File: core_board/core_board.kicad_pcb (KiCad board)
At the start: 2 copper layers, 101.6 x 113.2 mm, 111 parts, among them J1 Molex_Megafit_02, J10 Conn_01x04_Pin, J11 Conn_01x02_Pin, J12 Conn_01x02_Pin, J13 Conn_01x03_Pin, J14 Conn_01x02_Pin, J15 Conn_01x02_Pin, J16 Conn_01x03_Pin, J2 RJ45_LED_Shielded, J3 Conn_01x02_Pin, J4Serv1 Conn_01x04_Pin, J5 Conn_01x04_Pin, J6 Conn_01x02_Pin, J8 Conn_01x04_Pin, J9 Conn_01x02_Pin, Q1 TPC8132_LQS, Q18 BSS138, Q19 BSS138, Q2 BSS138, Q20 BSS138, Q21 BSS138, Q3 BSS138, Q4 BSS138, Q5 BSS138, Q6 BSS138, Q7 BSS138, SW1 SW_Push, SW2 SW_Push, SW3 SW_Push, SW4 SW_Push, U1 AP63301WU7, U4 BD9G401EFJ-E2

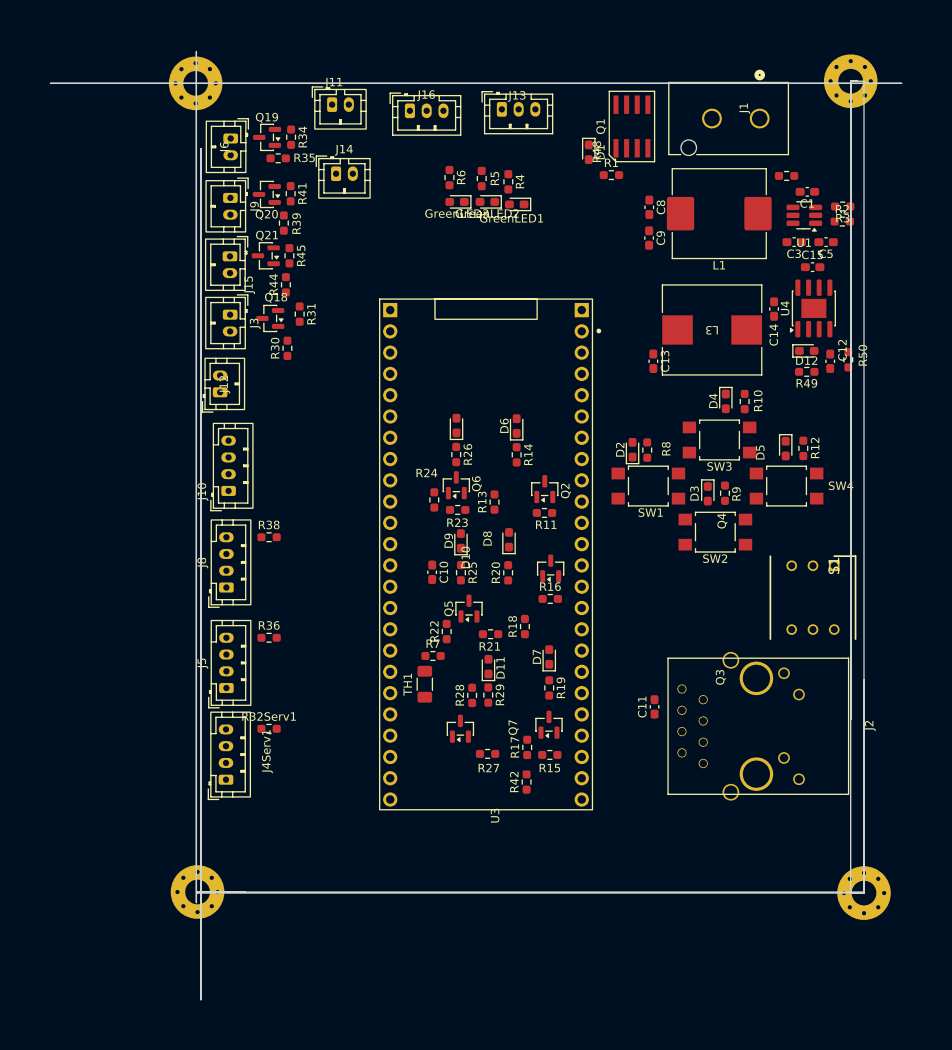
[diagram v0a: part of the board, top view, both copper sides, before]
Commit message: rough layout
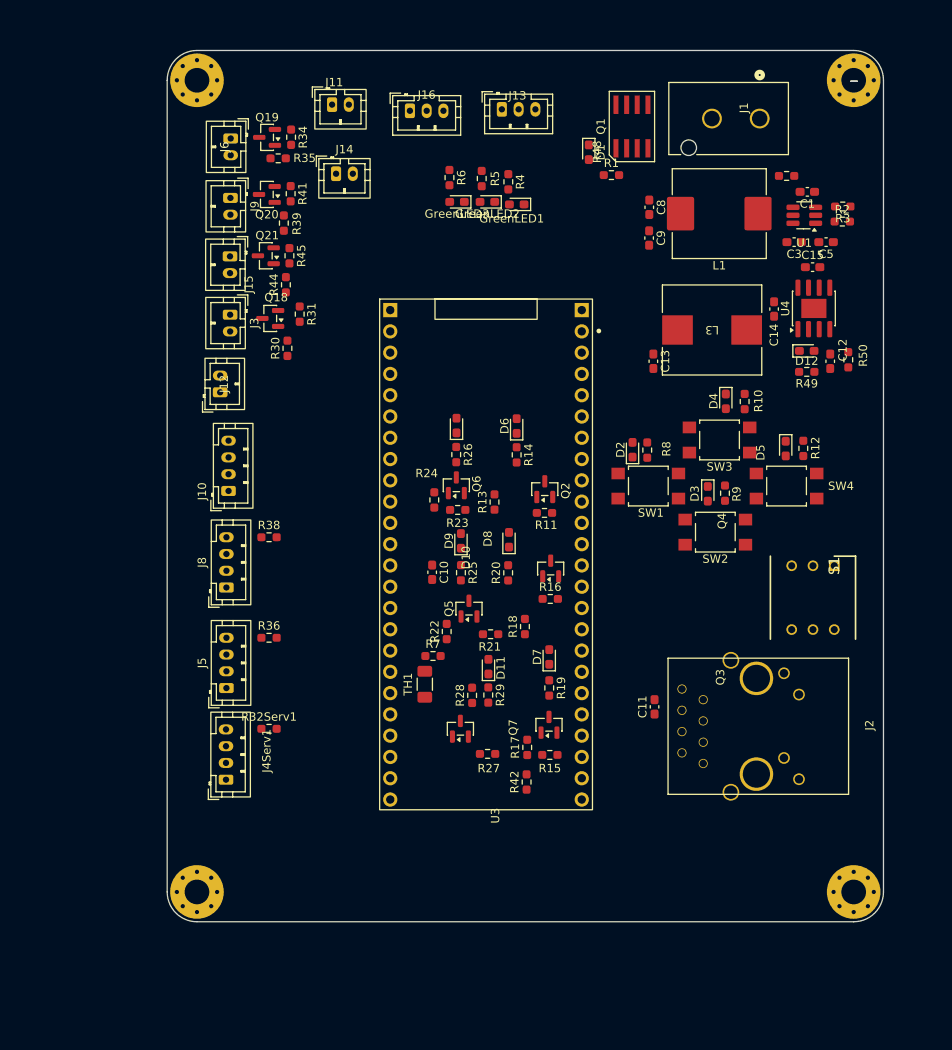
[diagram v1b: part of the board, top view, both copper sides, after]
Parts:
- moved U6 1.24 mm to (189.4, 123.4)
- moved U8 0.40 mm to (111.1, 26.6)
- moved U5 0.37 mm to (189.4, 26.6)
- moved U7 0.07 mm to (111.1, 123.4)
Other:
- board size 101.6 x 113.2 mm -> 85.5 x 104 mm
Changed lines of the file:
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@@
 	(footprint "MRDT_Drill_Holes:4_40_Hole_Pad_Via"
 		(layer "F.Cu")
-		(at 189.09 26.67)
+		(at 189.444 26.556)
 		(property "Reference" "U5"
 			(at 0 -0.5 0)
@@
 	(footprint "MRDT_Drill_Holes:4_40_Hole_Pad_Via"
 		(layer "F.Cu")
-		(at 190.677944 123.577944)
+		(at 189.444 123.444)
 		(property "Reference" "U6"
 			(at 0 -0.5 0)
@@
 	(footprint "MRDT_Drill_Holes:4_40_Hole_Pad_Via"
 		(layer "F.Cu")
-		(at 111.125 123.45)
+		(at 111.056 123.444)
 		(property "Reference" "U7"
 			(at 0 -0.5 0)
@@
 	(footprint "MRDT_Drill_Holes:4_40_Hole_Pad_Via"
 		(layer "F.Cu")
-		(at 110.9 26.925)
+		(at 111.056 26.556)
 		(property "Reference" "U8"
 			(at 0 -0.5 0)
@@
 		)
 	)
-	(gr_rect
-		(start 93.568944 26.925)
-		(end 195.168944 26.925)
+	(gr_arc
+		(start 107.5 26.556)
+		(mid 108.541528 24.041528)
+		(end 111.056 23)
 		(stroke
 			(width 0.05)
 			(type default)
 		)
-		(fill no)
 		(layer "Edge.Cuts")
 	)
-	(gr_rect
-		(start 110.985 23.12)
-		(end 110.985 124.72)
+	(gr_line
+		(start 107.5 123.444)
+		(end 107.5 26.556)
 		(stroke
 			(width 0.05)
 			(type default)
 		)
-		(fill no)
 		(layer "Edge.Cuts")
 	)
-	(gr_rect
-		(start 111.125 123.45)
-		(end 116.84 123.45)
+	(gr_line
+		(start 111.056 23)
+		(end 189.444 23)
 		(stroke
 			(width 0.05)
 			(type default)
 		)
-		(fill no)
 		(layer "Edge.Cuts")
 	)
-	(gr_rect
-		(start 111.125 123.45)
-		(end 190.677944 123.577944)
+	(gr_arc
+		(start 111.056 127)
+		(mid 108.541528 125.958472)
+		(end 107.5 123.444)
 		(stroke
 			(width 0.05)
 			(type default)
 		)
-		(fill no)
 		(layer "Edge.Cuts")
 	)
 	(gr_rect
-		(start 111.526856 34.717344)
-		(end 111.526856 136.317344)
+		(start 189.09 26.67)
+		(end 189.883972 26.67)
 		(stroke
 			(width 0.05)
@@
 		(layer "Edge.Cuts")
 	)
-	(gr_rect
-		(start 189.09 26.67)
-		(end 189.09 102.87)
+	(gr_arc
+		(start 189.444 23)
+		(mid 191.958472 24.041528)
+		(end 193 26.556)
 		(stroke
 			(width 0.05)
 			(type default)
 		)
-		(fill no)
 		(layer "Edge.Cuts")
 	)
-	(gr_rect
-		(start 189.09 26.67)
-		(end 189.883972 26.67)
+	(gr_line
+		(start 189.444 127)
+		(end 111.056 127)
 		(stroke
 			(width 0.05)
 			(type default)
 		)
-		(fill no)
 		(layer "Edge.Cuts")
 	)
-	(gr_rect
-		(start 189.09 26.67)
-		(end 190.677944 123.577944)
+	(gr_line
+		(start 193 26.556)
+		(end 193 123.444)
 		(stroke
 			(width 0.05)
 			(type default)
 		)
-		(fill no)
 		(layer "Edge.Cuts")
 	)
-	(gr_rect
-		(start 190.677944 98.177944)
-		(end 190.677944 123.577944)
+	(gr_arc
+		(start 193 123.444)
+		(mid 191.958472 125.958472)
+		(end 189.444 127)
 		(stroke
 			(width 0.05)
 			(type default)
 		)
-		(fill no)
 		(layer "Edge.Cuts")
 	)
